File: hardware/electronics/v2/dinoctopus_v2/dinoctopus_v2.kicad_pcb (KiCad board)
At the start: 2 copper layers, 60 x 70 mm, 68 parts, among them J1 Conn_01x04_Socket, J1-I1 SJ-3524-SMT, J1-I2 SJ-3524-SMT, J1-I3 SJ-3524-SMT, J1-I4 SJ-3524-SMT, J1-I5 SJ-3524-SMT, J11-O1 SJ-3524-SMT, J11-O2 SJ-3524-SMT, J11-O3 SJ-3524-SMT, J11-O4 SJ-3524-SMT, J11-O5 SJ-3524-SMT, J2 Conn_01x03_Pin, J3 Conn_01x05_Pin, J4 Conn_01x05_Pin, J5 Conn_01x03_Pin, J6 Conn_01x04_Pin, J7 Conn_01x03_Pin, U1 Pico mounting, U2 H11L1, U3 H11L1, U4 H11L1, U5 H11L1, U6 H11L1

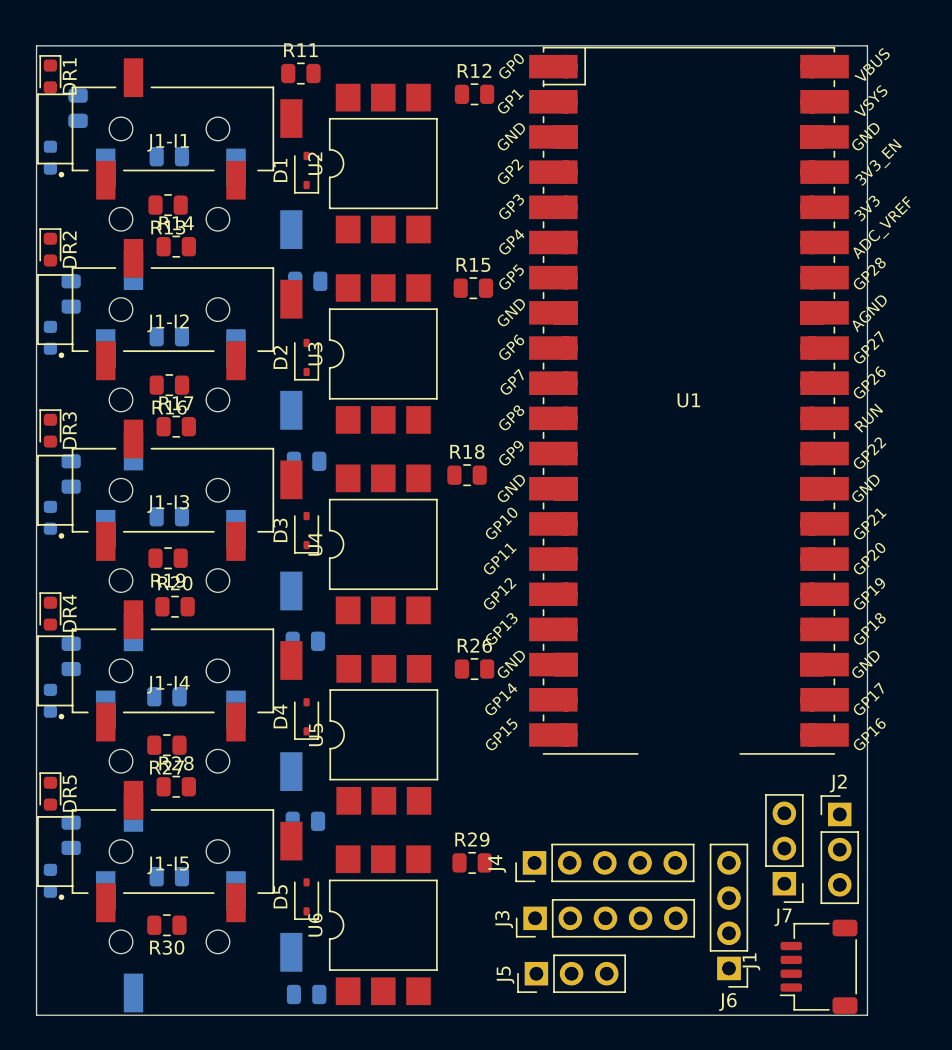
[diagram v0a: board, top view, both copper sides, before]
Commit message: giant mess
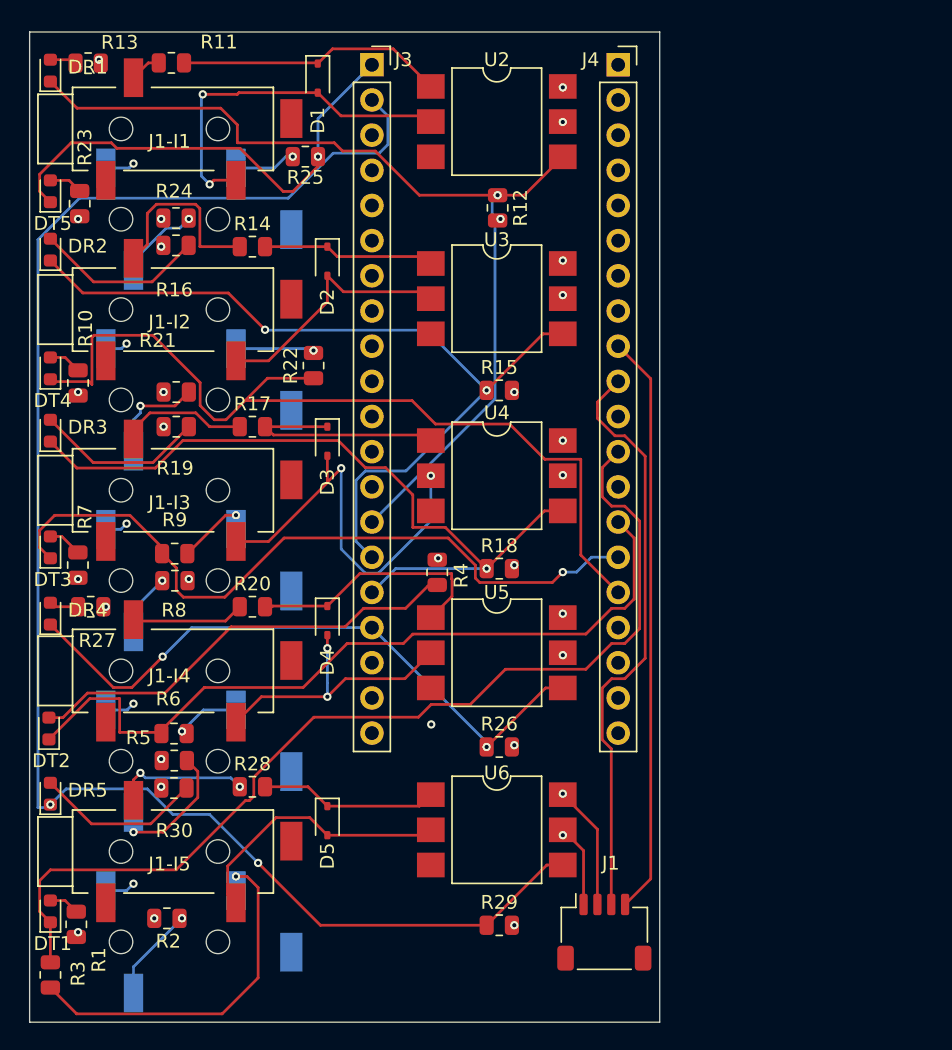
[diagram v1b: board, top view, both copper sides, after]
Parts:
- removed J2, J5, J7: Conn_01x03_Pin, Connector_PinHeader_2.54mm:PinHeader_1x03_P2.54mm_Vertical
- removed J6: Conn_01x04_Pin, Connector_PinHeader_2.54mm:PinHeader_1x04_P2.54mm_Vertical
- removed U1: Pico mounting, Library:RPi_Pico_SMD_Only
- DR1, DR2, DR3, DR4, DR5: footprint LED_SMD:LED_0603_1608Metric -> Library:rx_with_light_pipe
- DT1, DT2, DT3, DT4, DT5: footprint LED_SMD:LED_0603_1608Metric -> Library:tx_with_light_pipe; moved to F.Cu
- J3, J4: value Conn_01x05_Pin -> Conn_01x20_Pin; footprint Connector_PinHeader_2.54mm:PinHeader_1x05_P2.54mm_Vertical -> Connector_PinSocket_2.54mm:PinSocket_1x20_P2.54mm_Vertical
- R1, R10, R2, R21, R22, R23, R24, R25, R3, R4, R5, R6, R7, R8, R9: moved to F.Cu
- moved J3 62.8 mm to (51.2, 31.9), turned to 0 degrees
- moved J4 57.9 mm to (69.0, 31.9), turned to 0 degrees
- moved R4 27.1 mm to (55.9, 68.5)
- moved J1 15.7 mm to (68.0, 94.5), turned to 0 degrees
- moved R13 11.8 mm to (30.7, 31.8)
- moved R2 11.5 mm to (36.4, 93.5), turned to 0 degrees
- moved R27 11.4 mm to (30.9, 71.0)
- moved R3 11.1 mm to (28.0, 97.6), turned to -90 degrees
- moved U6 10.7 mm to (60.2, 87.1), turned to 0 degrees
- moved R21 10.7 mm to (37.1, 55.5), turned to 0 degrees
- moved R22 10.6 mm to (47.0, 53.6), turned to 90 degrees
- moved R24 10.6 mm to (37.1, 42.9), turned to 0 degrees
- moved R5 10.4 mm to (36.9, 82.1), turned to 0 degrees
- moved R8 10.4 mm to (37.0, 69.1)
- moved R16 10.1 mm to (37.1, 44.9), turned to 0 degrees
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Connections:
- J3 pad 1: Net-(J3-Pin_1) -> /Midi Output 5/TX
- J3 pad 2: Net-(J3-Pin_2) -> /MIDI input 5/RX
- J4 pad 3: Net-(J4-Pin_3) -> GND
- J4 pad 5: Net-(J4-Pin_5) -> +3V3
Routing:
- net /MIDI input 5/RX: track 0.00 -> 117.2 mm, vias 0 -> 2
- net /Midi Output 1/TX: track 0.00 -> 72.8 mm
- net /MIDI input 1/RX: track 0.00 -> 69.8 mm, vias 0 -> 1
- net /Midi Output 4/TX: track 0.00 -> 64.1 mm
- net /MIDI input 2/RX: track 0.00 -> 60.7 mm, vias 0 -> 2
- net /Midi Output 2/TX: track 0.00 -> 55.9 mm
- net /MIDI input 3/RX: track 0.00 -> 54.5 mm, vias 0 -> 1
- net /Midi Output 3/TX: track 0.00 -> 52.6 mm, vias 0 -> 1
- net /MIDI input 4/RX: track 0.00 -> 46.2 mm, vias 0 -> 2
- net Net-(J1-Pin_3): track 0.00 -> 42.4 mm
- net Net-(J1-Pin_4): track 0.00 -> 42.1 mm
- net /Midi Output 5/TX: track 0.00 -> 34.9 mm, vias 0 -> 1
- net Net-(DT2-A): track 0.00 -> 32.0 mm
- net Net-(D3-A): track 0.00 -> 29.6 mm, vias 0 -> 2
- net Net-(D1-A): track 0.00 -> 26.2 mm, vias 0 -> 2
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- added copper zone on In1.Cu, net +3V3
- added copper zone on In2.Cu, net GND
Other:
- board size 60 x 70 mm -> 45.5 x 71.5 mm
- copper layers 2 -> 4
- board text added: "JLCJLCJLCJLC"
- board text added: "dinoctopus - rev 2 bjonnh-midi@bjonnh.net"
